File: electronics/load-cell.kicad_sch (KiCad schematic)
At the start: 21 parts, among them J1 Conn_01x03, J2 Conn_01x03, J3 Conn_01x03, J4 Conn_01x03, Q4 PNP, U1 HX711, U7 TPS7A0533PDBV

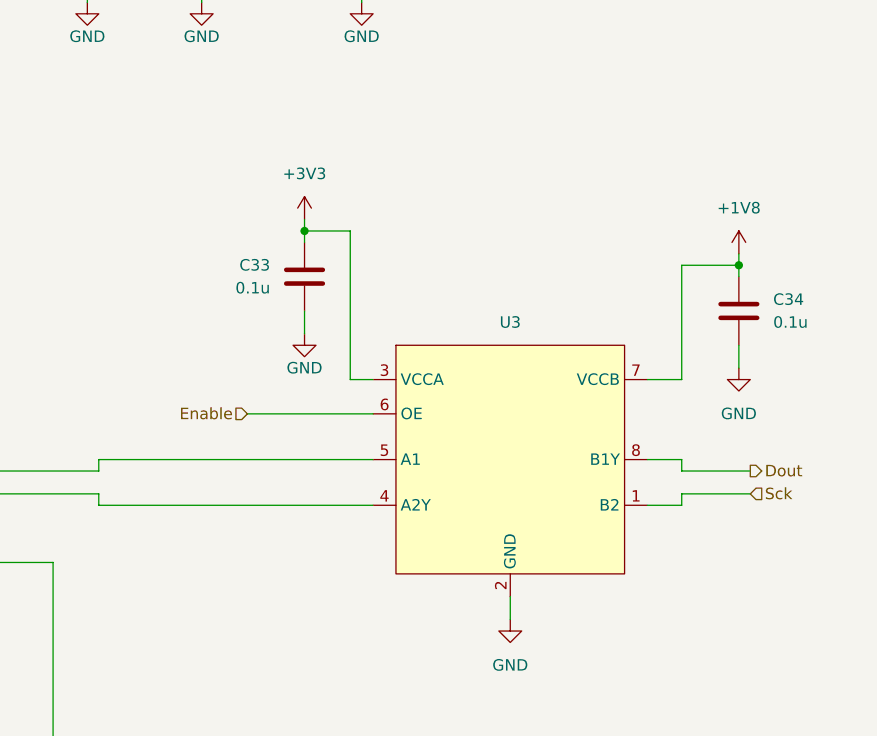
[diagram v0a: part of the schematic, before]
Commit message: electronics: initial placement
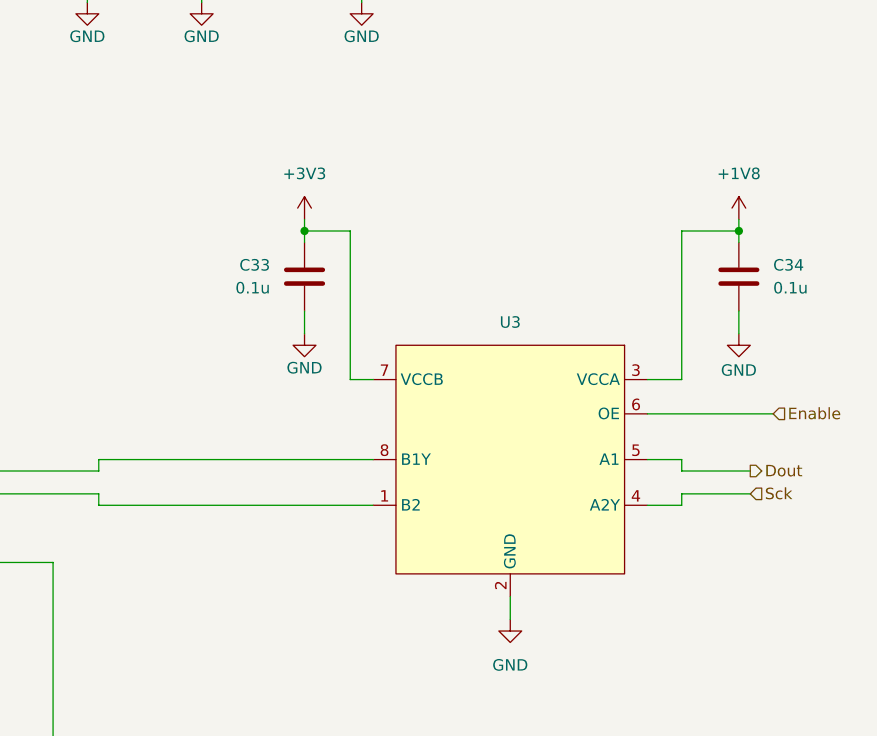
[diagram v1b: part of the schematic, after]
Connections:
- net +1V8: now also U3.3 (VCCA); no longer U3.7 (VCCB)
- net +3V3: now also U3.7 (VCCB); no longer U3.3 (VCCA)
- net Dout: now also U3.5 (A1); no longer U3.8 (B1Y)
- net Sck: now also U3.4 (A2Y); no longer U3.1 (B2)
- net at U1.11 (PD_SCK): now also U3.1 (B2); no longer U3.4 (A2Y)
- net at U1.12 (DOUT): now also U3.8 (B1Y); no longer U3.5 (A1)
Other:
- moved on the sheet: C34
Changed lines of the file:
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@@
 	)
 	(junction
-		(at 294.64 62.23)
+		(at 294.64 58.42)
 		(diameter 0)
 		(color 0 0 0 0)
@@
 	(wire
 		(pts
-			(xy 240.03 78.74) (xy 254 78.74)
+			(xy 298.45 78.74) (xy 284.48 78.74)
 		)
 		(stroke
@@
 	(wire
 		(pts
-			(xy 294.64 71.12) (xy 294.64 73.66)
+			(xy 294.64 67.31) (xy 294.64 69.85)
 		)
 		(stroke
@@
 	(wire
 		(pts
-			(xy 294.64 62.23) (xy 294.64 63.5)
+			(xy 294.64 58.42) (xy 294.64 59.69)
 		)
 		(stroke
@@
 	(wire
 		(pts
-			(xy 288.29 74.93) (xy 288.29 62.23)
+			(xy 288.29 74.93) (xy 288.29 58.42)
 		)
 		(stroke
@@
 	(wire
 		(pts
-			(xy 294.64 60.96) (xy 294.64 62.23)
+			(xy 294.64 57.15) (xy 294.64 58.42)
 		)
 		(stroke
@@
 	(wire
 		(pts
-			(xy 288.29 62.23) (xy 294.64 62.23)
+			(xy 288.29 58.42) (xy 294.64 58.42)
 		)
 		(stroke
@@
 	(hierarchical_label "Enable"
 		(shape input)
-		(at 240.03 78.74 180)
+		(at 298.45 78.74 0)
 		(effects
 			(font
 				(size 1.27 1.27)
 			)
-			(justify right)
+			(justify left)
 		)
 	)
@@
 	(symbol
 		(lib_id "Device:C")
-		(at 294.64 67.31 0)
+		(at 294.64 63.5 0)
 		(unit 1)
 		(body_style 1)
@@
 		(dnp no)
 		(property "Reference" "C34"
-			(at 298.45 66.0399 0)
+			(at 298.45 62.2299 0)
 			(show_name no)
 			(do_not_autoplace no)
@@
 		)
 		(property "Value" "0.1u"
-			(at 298.45 68.5799 0)
+			(at 298.45 64.7699 0)
 			(show_name no)
 			(do_not_autoplace no)
@@
 		)
 		(property "Footprint" "Capacitor_SMD:C_0603_1608Metric"
-			(at 295.6052 71.12 0)
+			(at 295.6052 67.31 0)
 			(hide yes)
 			(show_name no)
@@
 		)
 		(property "Datasheet" ""
-			(at 294.64 67.31 0)
+			(at 294.64 63.5 0)
 			(hide yes)
 			(show_name no)
@@
 		)
 		(property "Description" "Unpolarized capacitor"
-			(at 294.64 67.31 0)
+			(at 294.64 63.5 0)
 			(hide yes)
 			(show_name no)
@@
 	(symbol
 		(lib_id "power:+1V8")
-		(at 294.64 60.96 0)
+		(at 294.64 57.15 0)
 		(unit 1)
 		(body_style 1)
@@
 		(fields_autoplaced yes)
 		(property "Reference" "#PWR08"
-			(at 294.64 64.77 0)
+			(at 294.64 60.96 0)
 			(hide yes)
 			(show_name no)
@@
 		)
 		(property "Value" "+1V8"
-			(at 294.64 55.88 0)
+			(at 294.64 52.07 0)
 			(show_name no)
 			(do_not_autoplace no)
@@
 		)
 		(property "Footprint" ""
-			(at 294.64 60.96 0)
+			(at 294.64 57.15 0)
 			(hide yes)
 			(show_name no)
@@
 		)
 		(property "Datasheet" ""
-			(at 294.64 60.96 0)
+			(at 294.64 57.15 0)
 			(hide yes)
 			(show_name no)
@@
 		)
 		(property "Description" "Power symbol creates a global label with name \"+1V8\""
-			(at 294.64 60.96 0)
+			(at 294.64 57.15 0)
 			(hide yes)
 			(show_name no)
@@
 		(lib_id "MyScale:TXU0202")
 		(at 269.24 83.82 0)
+		(mirror y)
 		(unit 1)
 		(body_style 1)
@@
 		(in_pos_files yes)
 		(dnp no)
-		(fields_autoplaced yes)
 		(property "Reference" "U3"
 			(at 269.24 68.58 0)
@@
 	(symbol
 		(lib_id "power:GND")
-		(at 294.64 73.66 0)
+		(at 294.64 69.85 0)
 		(mirror y)
 		(unit 1)
@@
 		(in_pos_files yes)
 		(dnp no)
-		(fields_autoplaced yes)
 		(property "Reference" "#PWR061"
-			(at 294.64 80.01 0)
+			(at 294.64 76.2 0)
 			(hide yes)
 			(show_name no)
@@
 		)
 		(property "Value" "GND"
-			(at 294.64 78.74 0)
+			(at 294.64 73.914 0)
 			(show_name no)
 			(do_not_autoplace no)
@@
 		)
 		(property "Footprint" ""
-			(at 294.64 73.66 0)
+			(at 294.64 69.85 0)
 			(hide yes)
 			(show_name no)
@@
 		)
 		(property "Datasheet" ""
-			(at 294.64 73.66 0)
+			(at 294.64 69.85 0)
 			(hide yes)
 			(show_name no)
@@
 		)
 		(property "Description" "Power symbol creates a global label with name \"GND\" , ground"
-			(at 294.64 73.66 0)
+			(at 294.64 69.85 0)
 			(hide yes)
 			(show_name no)
